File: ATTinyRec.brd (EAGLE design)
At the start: 15.7 x 29.3 mm, 10 parts, among them IC1 MAX631CPA, IC2 REG1117, M1 ELECTRET_MICROPHON-WM-62PC/62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, U1 ATTINY85-20SU, U2 USD-SOCKETUSD

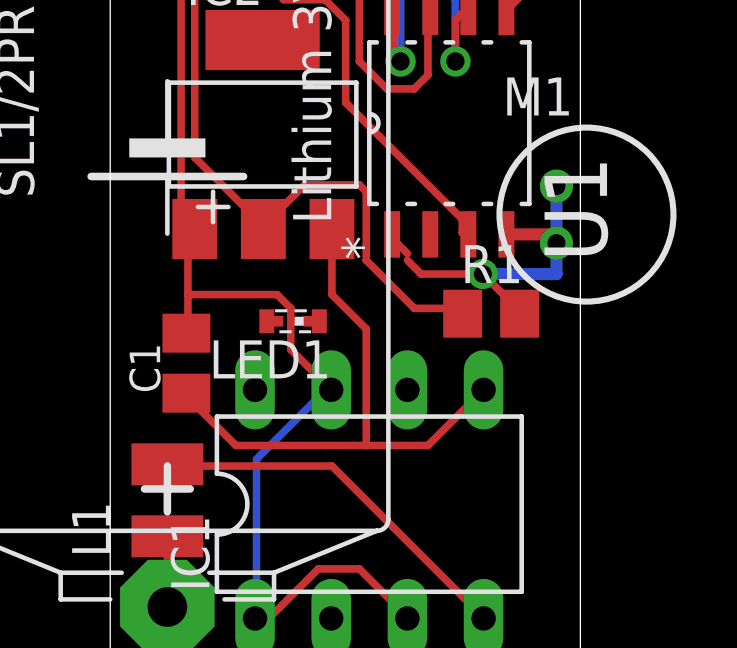
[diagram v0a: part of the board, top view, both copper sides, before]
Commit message: Debugging
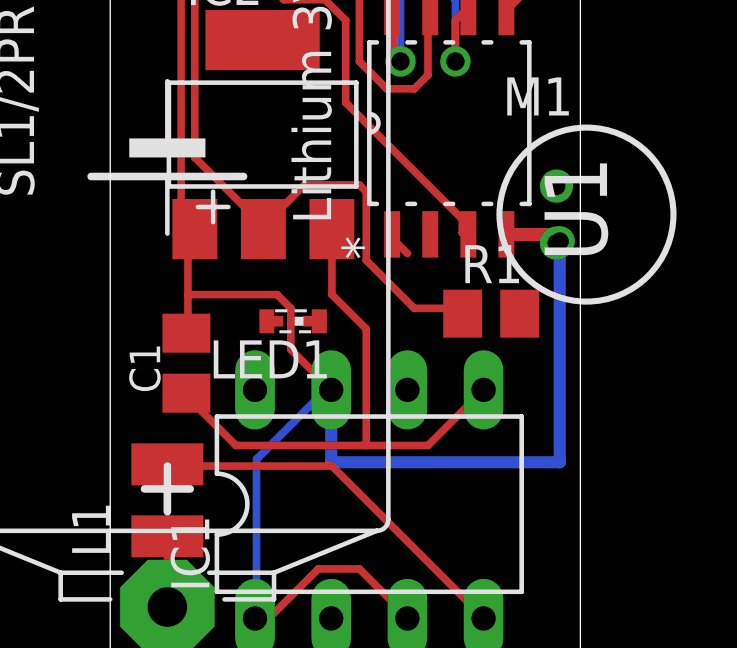
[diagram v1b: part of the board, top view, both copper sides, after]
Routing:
- net N$10: track 50.1 -> 69.5 mm, vias 0 -> 1
- net N$8: track 9.90 -> 0.00 mm, vias 1 -> 0
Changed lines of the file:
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@@
 <contactref element="M1" pad="1"/>
 <contactref element="R1" pad="2"/>
-<wire x1="14.1732" y1="25.8318" x2="13.716" y2="26.289" width="0.254" layer="1"/>
-<wire x1="16.2306" y1="25.8318" x2="14.1732" y2="25.8318" width="0.254" layer="1"/>
-<wire x1="17.3736" y1="24.6888" x2="16.2306" y2="25.8318" width="0.254" layer="1"/>
-<wire x1="17.3736" y1="24.6888" x2="17.46" y2="24.511" width="0.254" layer="1"/>
-<via x="16.2306" y="25.8318" extent="1-16" drill="0.6"/>
-<wire x1="16.2306" y1="25.8318" x2="18.685" y2="25.8318" width="0.4064" layer="16"/>
-<wire x1="18.685" y1="25.8318" x2="18.685" y2="28.763" width="0.4064" layer="16"/>
+<wire x1="17.46" y1="24.511" x2="18.685" y2="28.763" width="0" layer="19" extent="1-1"/>
 </signal>
 <signal name="N$9">
@@
 <wire x1="9.8298" y1="23.3172" x2="9.8298" y2="24.6888" width="0.254" layer="1"/>
 <wire x1="11.176" y1="21.971" x2="9.8298" y2="23.3172" width="0.254" layer="1"/>
-<wire x1="9.8298" y1="24.6888" x2="17.018" y2="27.1526" width="0" layer="19" extent="1-1"/>
-<wire x1="9.406" y1="24.257" x2="9.8298" y2="24.6888" width="0" layer="19" extent="1-1"/>
+<wire x1="17.018" y1="27.1526" x2="18.796" y2="27.1526" width="0.4064" layer="1"/>
+<wire x1="18.796" y1="27.1526" x2="18.796" y2="26.924" width="0.4064" layer="1"/>
+<via x="18.796" y="26.924" extent="1-16" drill="0.6" shape="square"/>
+<wire x1="18.796" y1="26.924" x2="18.796" y2="19.558" width="0.4064" layer="16"/>
+<wire x1="18.796" y1="19.558" x2="11.176" y2="19.558" width="0.4064" layer="16"/>
+<wire x1="11.176" y1="19.558" x2="11.176" y2="21.971" width="0.4064" layer="16"/>
+<wire x1="9.8298" y1="24.6888" x2="9.406" y2="24.257" width="0" layer="19" extent="1-1"/>
 </signal>
 <signal name="N$11">
